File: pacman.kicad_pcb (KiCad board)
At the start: 2 copper layers, 227.4 x 78 mm, 150 parts, among them J1 RESET, J2 BOOT, SW1 MX_LED, SW10 MX_LED, SW11 MX_LED, SW12 MX_LED, SW13 MX_LED, SW14 MX_LED, SW15 MX_LED, SW16 MX_LED, SW17 MX_LED, SW18 MX_LED, SW19 MX_LED, SW2 MX_LED, SW20 MX_LED, SW21 MX_LED, SW22 MX_LED, SW23 MX_LED, SW24 MX_LED, SW25 MX_LED, SW26 MX_LED, SW27 MX_LED, SW28 MX_LED, SW29 MX_LED, SW3 MX_LED, SW30 MX_LED, SW31 MX_LED, SW32 MX_LED, SW33 MX_LED, SW34 MX_LED, SW35 MX_LED, SW36 MX_LED, SW37 MX_LED, SW38 MX_LED, SW39 MX_LED, SW4 MX_LED, SW40 MX_LED, SW41 MX_LED, SW42 RotaryEncoder_Switch, SW42_2 MX_LED, SW43 RotaryEncoder_Switch, SW44 MX_LED, SW45 MX_LED, SW46 MX_LED, SW47 MX_LED, SW48 MX_LED, SW5 MX_LED, SW6 MX_LED, SW7 MX_LED, SW8 MX_LED, SW9 MX_LED, U1 NCP1117-3.3_SOT223, U2 RP2040, U3 W25Q128JVS, Y1 12MHz

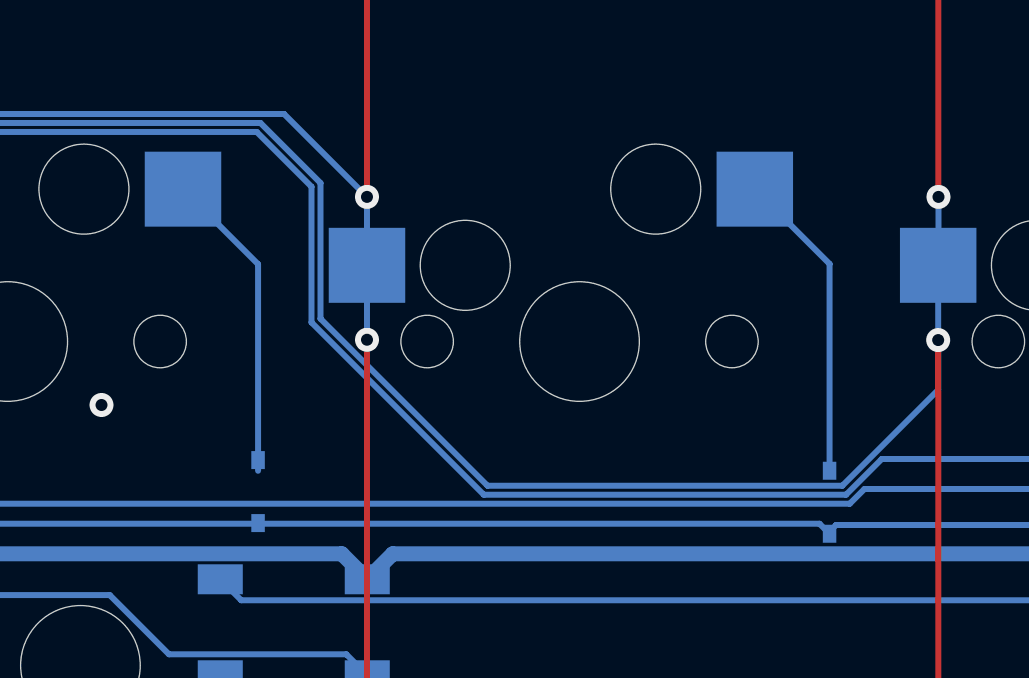
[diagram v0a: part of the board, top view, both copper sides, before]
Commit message: fix fill
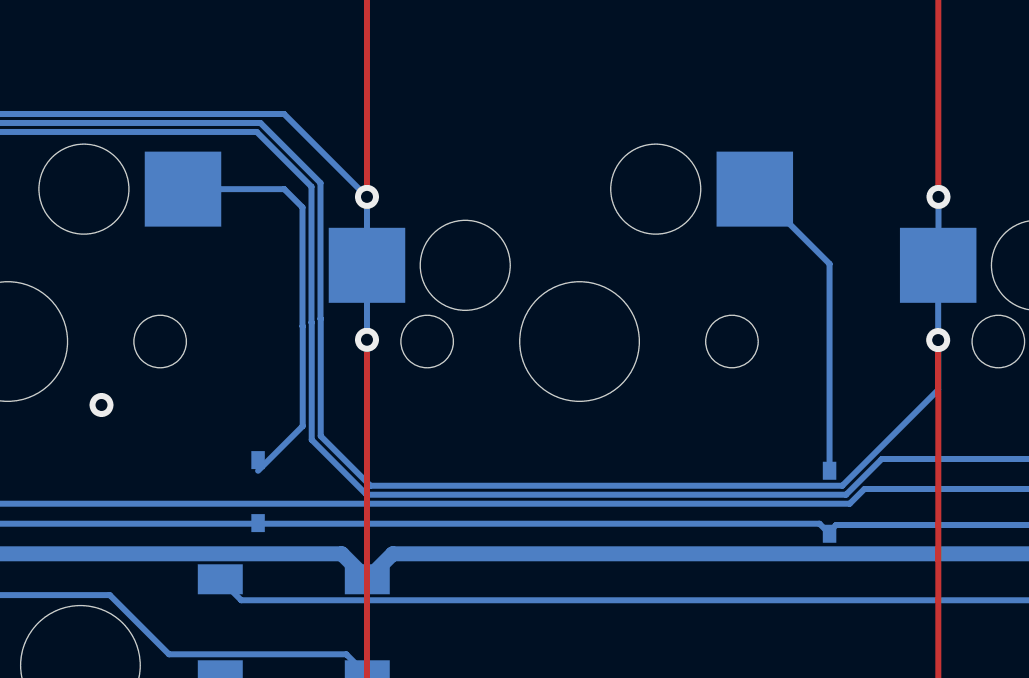
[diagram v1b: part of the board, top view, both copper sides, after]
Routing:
- net Net-(D31-A): track 10.4 -> 13.6 mm
- net col9: track 207.1 -> 209.4 mm
- net col8: track 187.1 -> 189.4 mm
